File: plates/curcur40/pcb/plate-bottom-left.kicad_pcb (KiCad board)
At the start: 2 copper layers, 116.1 x 88.3 mm, 0 parts

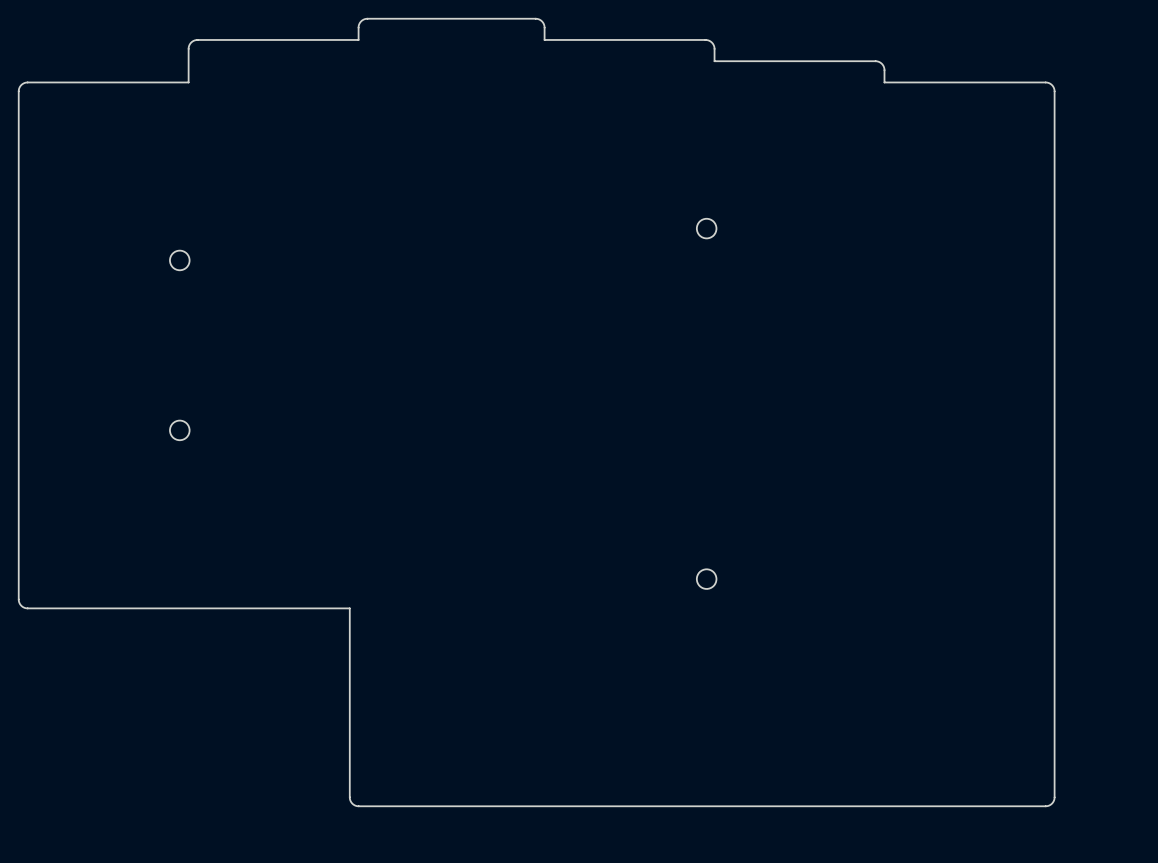
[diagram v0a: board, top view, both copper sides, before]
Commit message: fix all
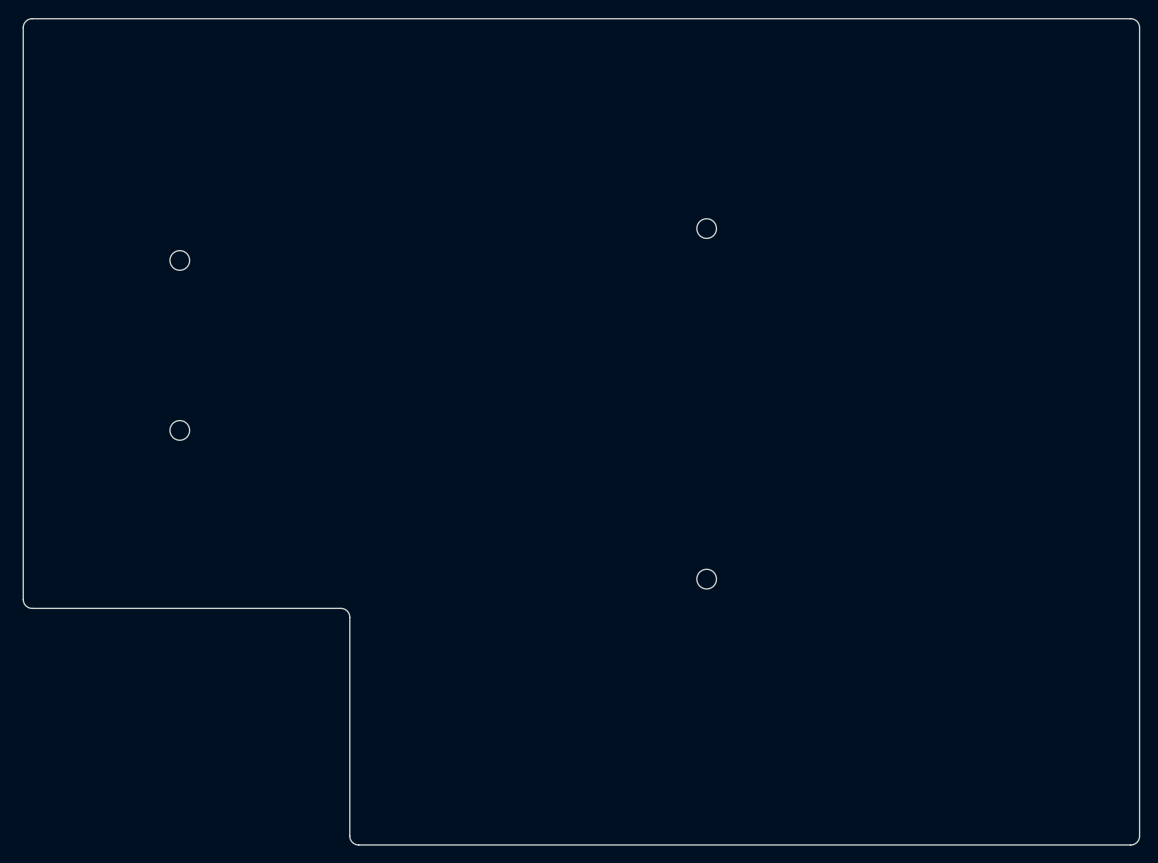
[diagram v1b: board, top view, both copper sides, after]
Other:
- board size 116.1 x 88.3 mm -> 125.1 x 92.6 mm
- rule pad_to_mask_clearance: 0.2 -> 0
